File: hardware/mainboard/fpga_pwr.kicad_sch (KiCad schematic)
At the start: 15 parts

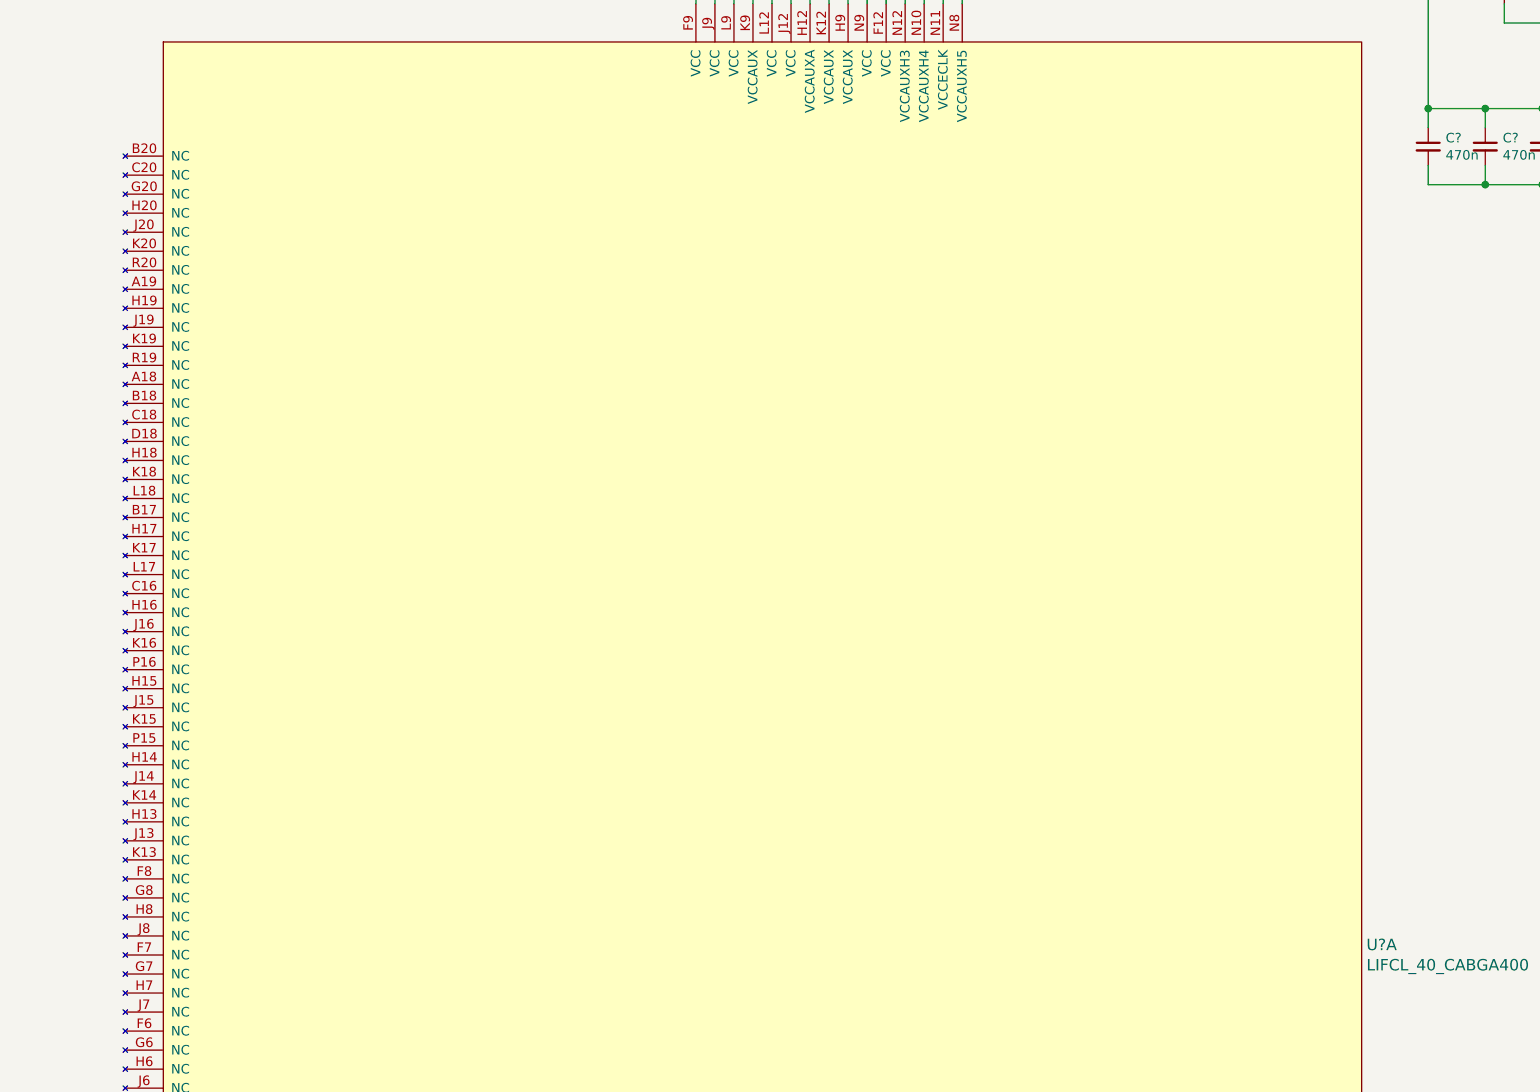
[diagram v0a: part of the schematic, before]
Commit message: Connecting up various bits
Signed-off-by: David Shah <dave@ds0.me>
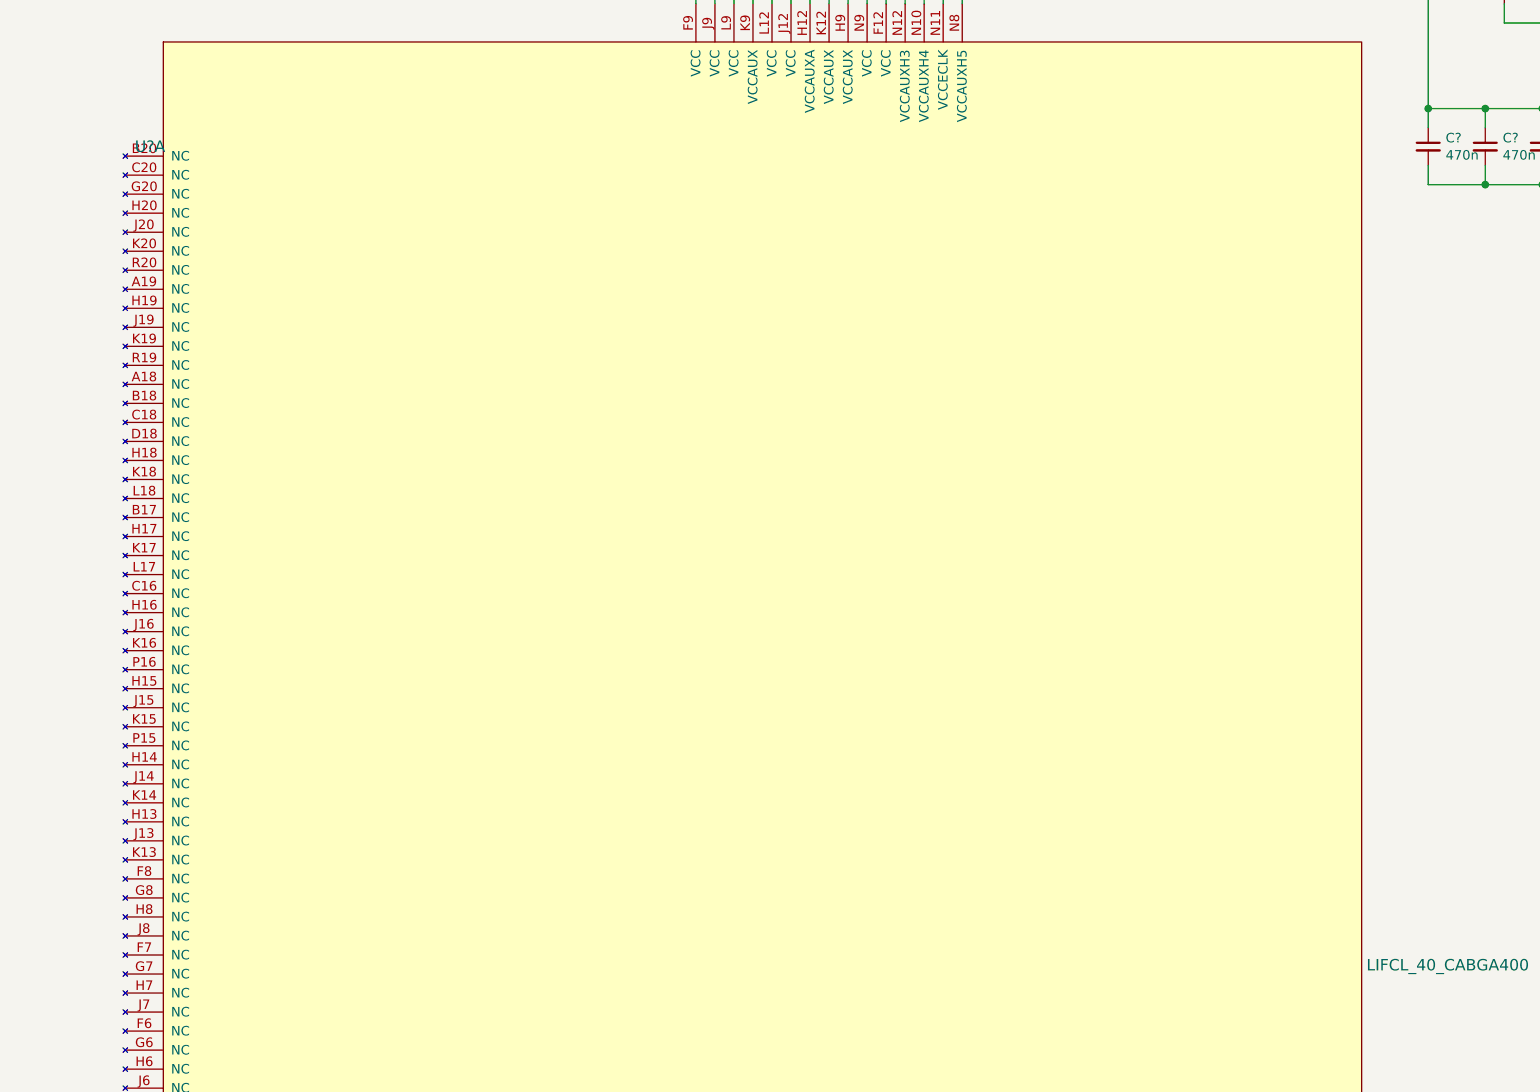
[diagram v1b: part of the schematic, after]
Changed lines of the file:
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@@
   (symbol (lib_id "meowality:LIFCL_40_CABGA400") (at 67.31 43.18 0) (unit 1)
     (in_bom yes) (on_board yes)
-    (property "Reference" "U?" (id 0) (at 233.0451 148.5062 0)
+    (property "Reference" "U?" (id 0) (at 68.58 41.91 0)
       (effects (font (size 1.524 1.524)) (justify left))
     )

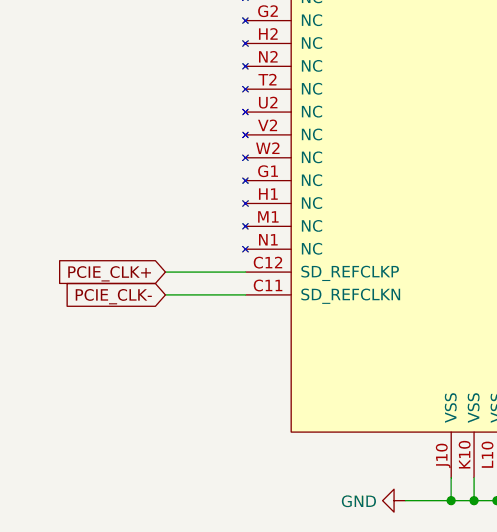
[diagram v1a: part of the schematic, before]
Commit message: More stuff
Signed-off-by: David Shah <dave@ds0.me>
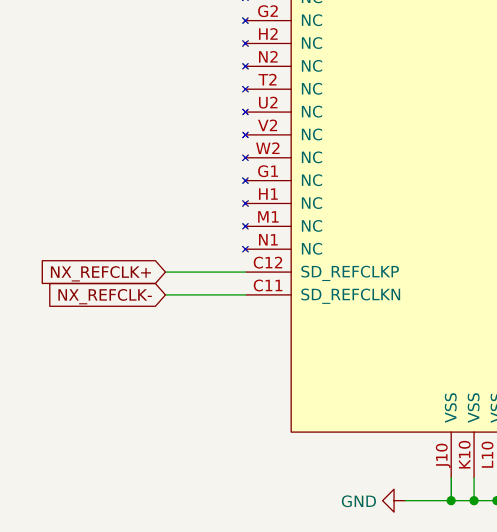
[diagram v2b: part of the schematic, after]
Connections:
- net PCIE_CLK+ renamed NX_REFCLK+
- net PCIE_CLK- renamed NX_REFCLK-
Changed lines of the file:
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@@
     (stroke (width 0) (type solid) (color 0 0 0 0))
   )
-  (global_label "PCIE_CLK+" (shape input) (at 58.42 254 180)
+  (global_label "NX_REFCLK+" (shape input) (at 58.42 254 180)
     (effects (font (size 1.27 1.27)) (justify right))
-    (property "Intersheet References" "${INTERSHEET_REFS}" (id 0) (at 44.081 253.9206 0)
+    (property "Intersheet References" "${INTERSHEET_REFS}" (id 0) (at 42.3272 254.0794 0)
       (effects (font (size 1.27 1.27)) (justify right) hide)
     )
   )
-  (global_label "PCIE_CLK-" (shape input) (at 58.42 256.54 180)
+  (global_label "NX_REFCLK-" (shape input) (at 58.42 256.54 180)
     (effects (font (size 1.27 1.27)) (justify right))
-    (property "Intersheet References" "${INTERSHEET_REFS}" (id 0) (at 44.081 256.4606 0)
+    (property "Intersheet References" "${INTERSHEET_REFS}" (id 0) (at 42.3272 256.6194 0)
       (effects (font (size 1.27 1.27)) (justify right) hide)
     )
